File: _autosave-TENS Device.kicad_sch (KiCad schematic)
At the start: 12 parts, among them SW1 SW_Push, U1 NE555P

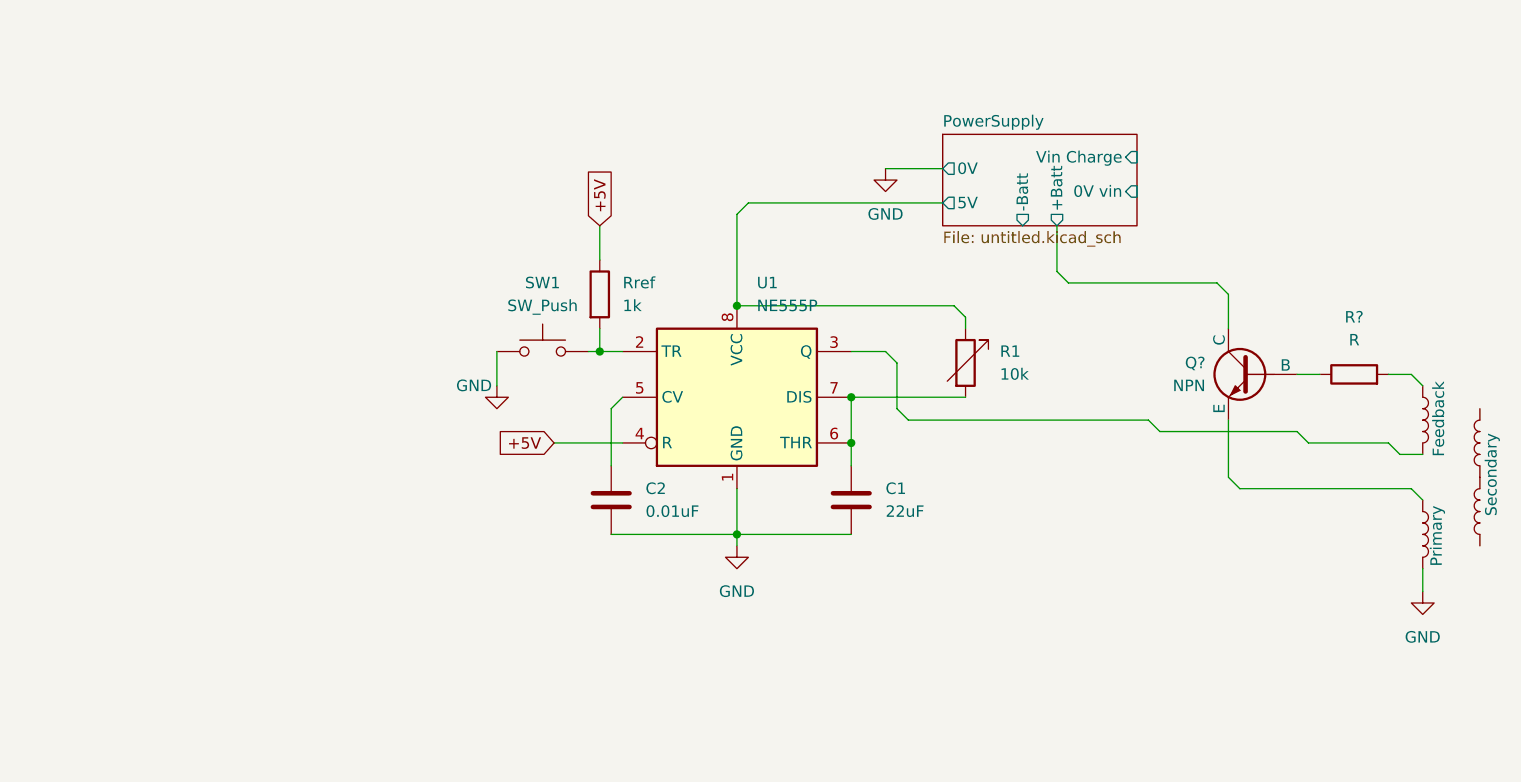
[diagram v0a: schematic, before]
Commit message: Backup
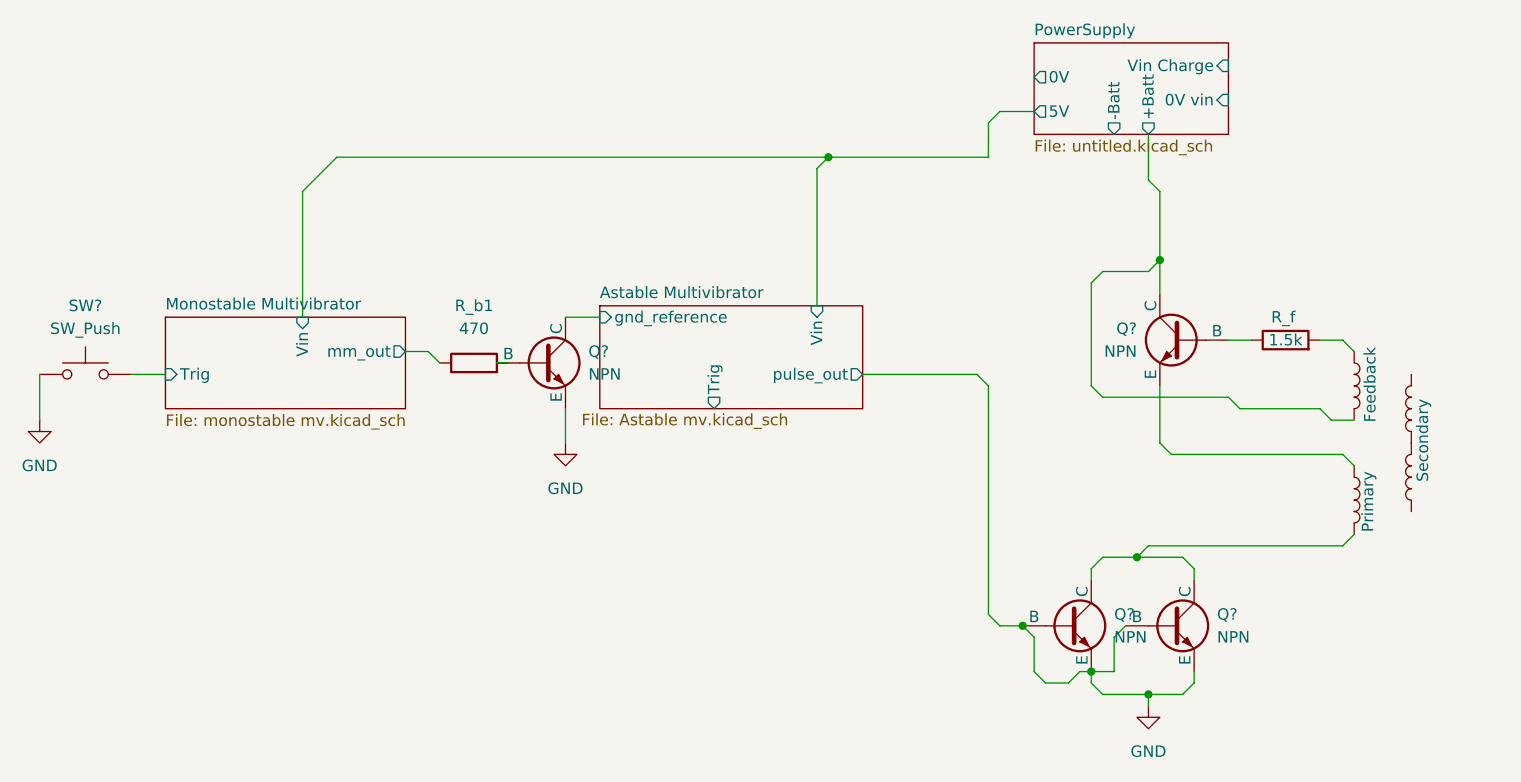
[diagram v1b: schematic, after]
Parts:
- removed C1: 22uF, symbol Device:C
- removed C2: 0.01uF, symbol Device:C
- removed R1: 10k, symbol Device:R_Variable
- removed Rref: 1k, symbol Device:R
- removed SW1: SW_Push, symbol Switch:SW_Push
- removed U1: NE555P, Package_DIP:DIP-8_W7.62mm, symbol Timer:NE555P
- added Q? (x3): NPN, symbol Simulation_SPICE:NPN
- added R_b1: 470, symbol Device:R
- added SW?: SW_Push, symbol Switch:SW_Push
- R_f: renamed from R?; value R -> 1.5k
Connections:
- net GND: now also Q?.2 (B), Q?.2 (B), Q?.3 (E), Q?.3 (E), Q?.3 (E), SW?.1; no longer Primary.2
- net PowerSupply/+Batt: now also Feedback.2
- new net: Q?.2 (B), R_b1.2
- new net: Primary.2, Q?.1 (C), Q?.1 (C)
- new net Astable Multivibrator/gnd_reference: Q?.1 (C)
- new net Monostable Multivibrator/Trig: SW?.2
- new net Monostable Multivibrator/mm_out: R_b1.1
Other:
- added sheet Astable Multivibrator (Astable mv.kicad_sch)
- added sheet Monostable Multivibrator (monostable mv.kicad_sch)
- moved on the sheet: Feedback, Primary, Q?, R_f, Secondary
